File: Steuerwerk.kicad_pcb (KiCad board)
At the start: 2 copper layers, 115 parts, among them J1 2PinTerminalBlocktg, J10 2PinTerminalBlocktg, J11 2PinTerminalBlocktg, J12 2PinTerminalBlocktg, J2 2PinTerminalBlocktg, J3 3PinTerminalBlocktg, J4 3PinTerminalBlocktg, J5 2PinTerminalBlocktg, J6 2PinTerminalBlocktg, J7 2PinTerminalBlocktg, J8 2PinTerminalBlocktg, J9 2PinTerminalBlocktg, Q1 Q_PNP_BCE, U1 74ls240, U2 74541, U3 74LS161, U4 74LS138, U5 74LS138, U6 74541, U7 74LS374, U8 74LS374

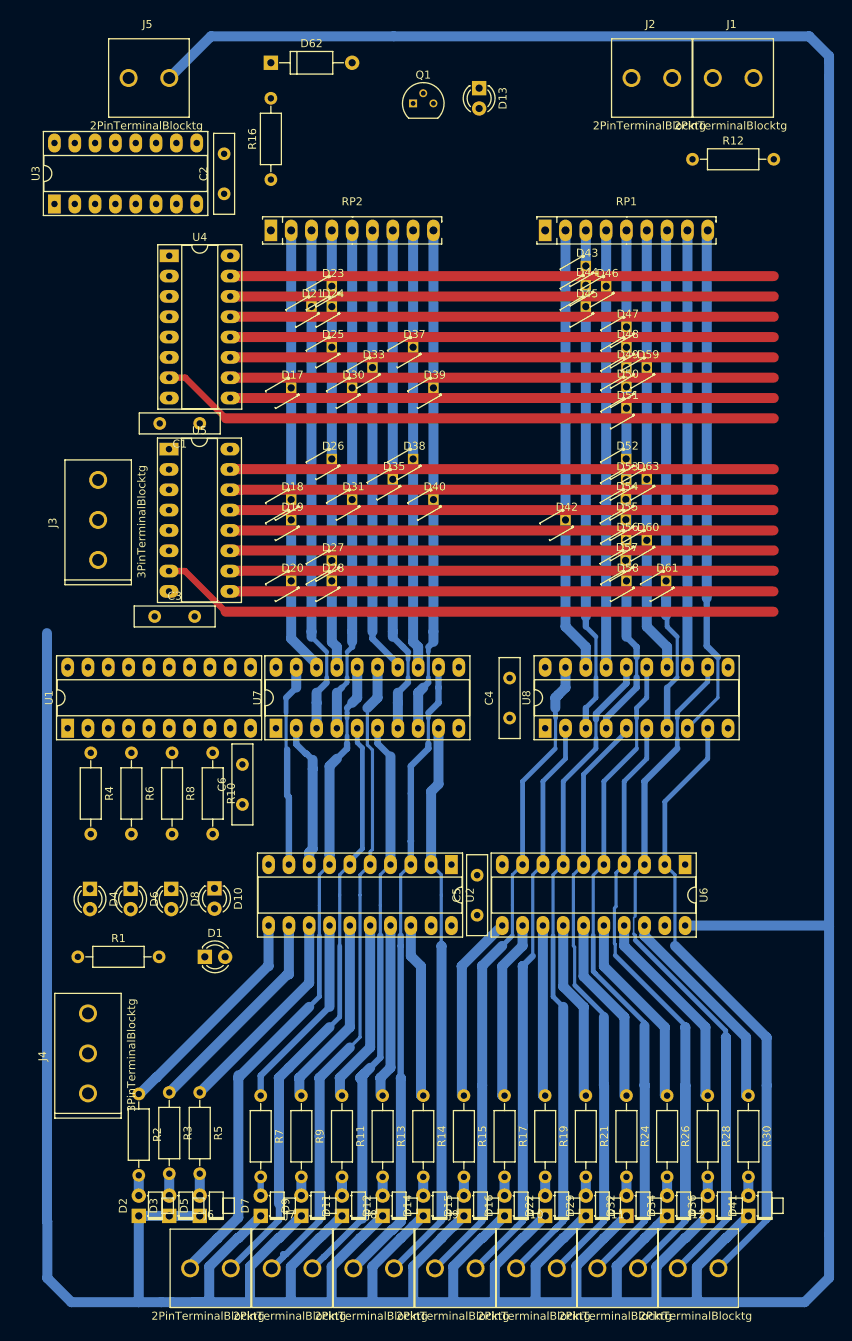
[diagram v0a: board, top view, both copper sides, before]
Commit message: steuerwerk improvements
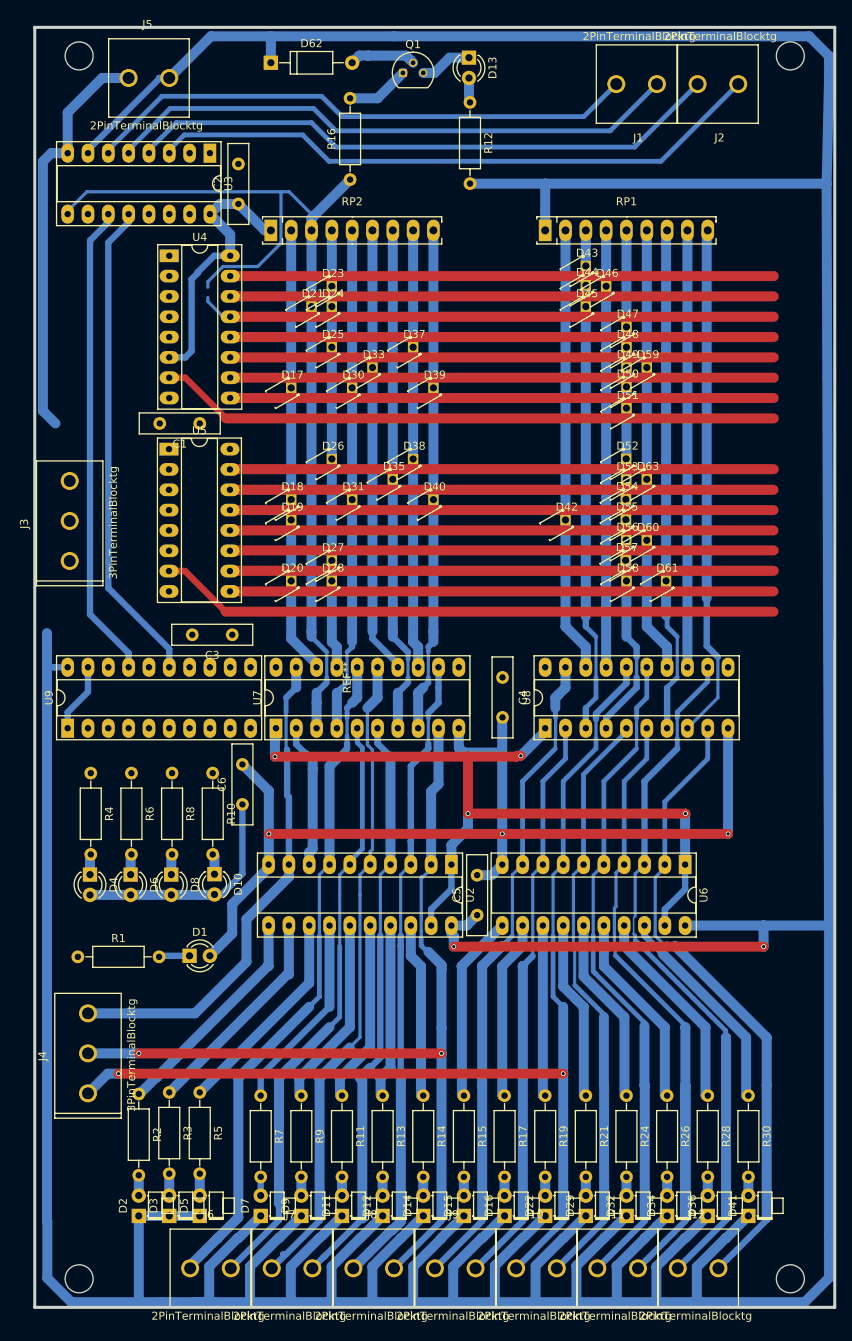
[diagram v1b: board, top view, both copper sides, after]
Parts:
- removed U1: 74ls240, Housings_DIP:DIP-20_W7.62mm_Socket_LongPads
- added REF**: EuroBoard160mmX100mm_holes, tg_foodprint:EuroBoard160mmX100mm_holes, F.Cu at (141.6, 193.6)
- added U9: 74ls240, Package_DIP:DIP-20_W7.62mm_Socket_LongPads, F.Cu at (45.8, 121.2)
- moved R12 28.7 mm to (96.0, 43.0), turned to 270 degrees
- moved U3 20.4 mm to (63.5, 49.4), turned to 270 degrees
- moved J1 12.1 mm to (116.9, 40.7), turned to 180 degrees
- moved C3 9.96 mm to (66.3, 109.6), turned to 180 degrees
- moved R16 9.91 mm to (81.1, 52.7)
- moved J2 8.29 mm to (127.0, 40.7), turned to 180 degrees
- moved C4 5.16 mm to (100.1, 114.9), turned to 270 degrees
- moved Q1 4.02 mm to (87.7, 39.3)
- moved D13 4.02 mm to (95.9, 37.4)
- moved J3 3.56 mm to (46.0, 95.3)
- moved R10 2.54 mm to (63.9, 126.9)
- moved R4 2.54 mm to (48.6, 126.9)
- moved R6 2.54 mm to (53.7, 126.9)
- moved R8 2.54 mm to (58.8, 126.9)
- moved C2 2.18 mm to (67.1, 55.7)
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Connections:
- D10 pad 1: (no net) -> Net-(D10-Pad1)
- D10 pad 2: (no net) -> VCC
- D4 pad 1: (no net) -> Net-(D4-Pad1)
- D4 pad 2: (no net) -> VCC
- D6 pad 1: (no net) -> Net-(D6-Pad1)
- D6 pad 2: (no net) -> VCC
- D8 pad 1: (no net) -> Net-(D8-Pad1)
- D8 pad 2: (no net) -> VCC
- R10 pad 2: (no net) -> Net-(D10-Pad1)
- R4 pad 2: (no net) -> Net-(D4-Pad1)
- R6 pad 2: (no net) -> Net-(D6-Pad1)
- R8 pad 2: (no net) -> Net-(D8-Pad1)
- U2 pad 1: (no net) -> /enSTW
- U2 pad 19: (no net) -> /enSTW
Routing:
- net GND: track 0.00 -> 197.6 mm, vias 0 -> 3
- net VCC: track 634.7 -> 816.0 mm, vias 0 -> 2
- net /enSTW: track 0.00 -> 104.4 mm, vias 0 -> 4
- net Net-(J2-Pad1): track 0.00 -> 77.7 mm
- net Net-(J2-Pad2): track 0.00 -> 74.9 mm
- net Net-(J1-Pad1): track 0.00 -> 72.2 mm
- net Net-(J1-Pad2): track 0.00 -> 69.4 mm
- net Net-(U3-Pad12): track 0.00 -> 60.9 mm
- net /11: track 82.7 -> 143.1 mm, vias 0 -> 2
- net /a2: track 63.8 -> 123.8 mm
- net Net-(U3-Pad11): track 0.00 -> 59.6 mm
- net /enAkku: track 70.9 -> 116.4 mm, vias 0 -> 2
- net /clrMPC: track 25.3 -> 62.2 mm
- net Net-(Q1-Pad1): track 0.00 -> 7.92 mm
- net Net-(D13-Pad1): track 0.00 -> 6.50 mm
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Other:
- board outline added: 100 x 160 mm
